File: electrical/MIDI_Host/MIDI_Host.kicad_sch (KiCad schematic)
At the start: 9 parts, among them CN1 USB-CON-AF-LCP-Offset, J1 Blackheadphonejack, J2 Blackheadphonejack, J3 USB_C_TYPE-C-32-M-12, SW1 ST-0-102-C03-N003-RS, SW2 TC-1109DE-C-G

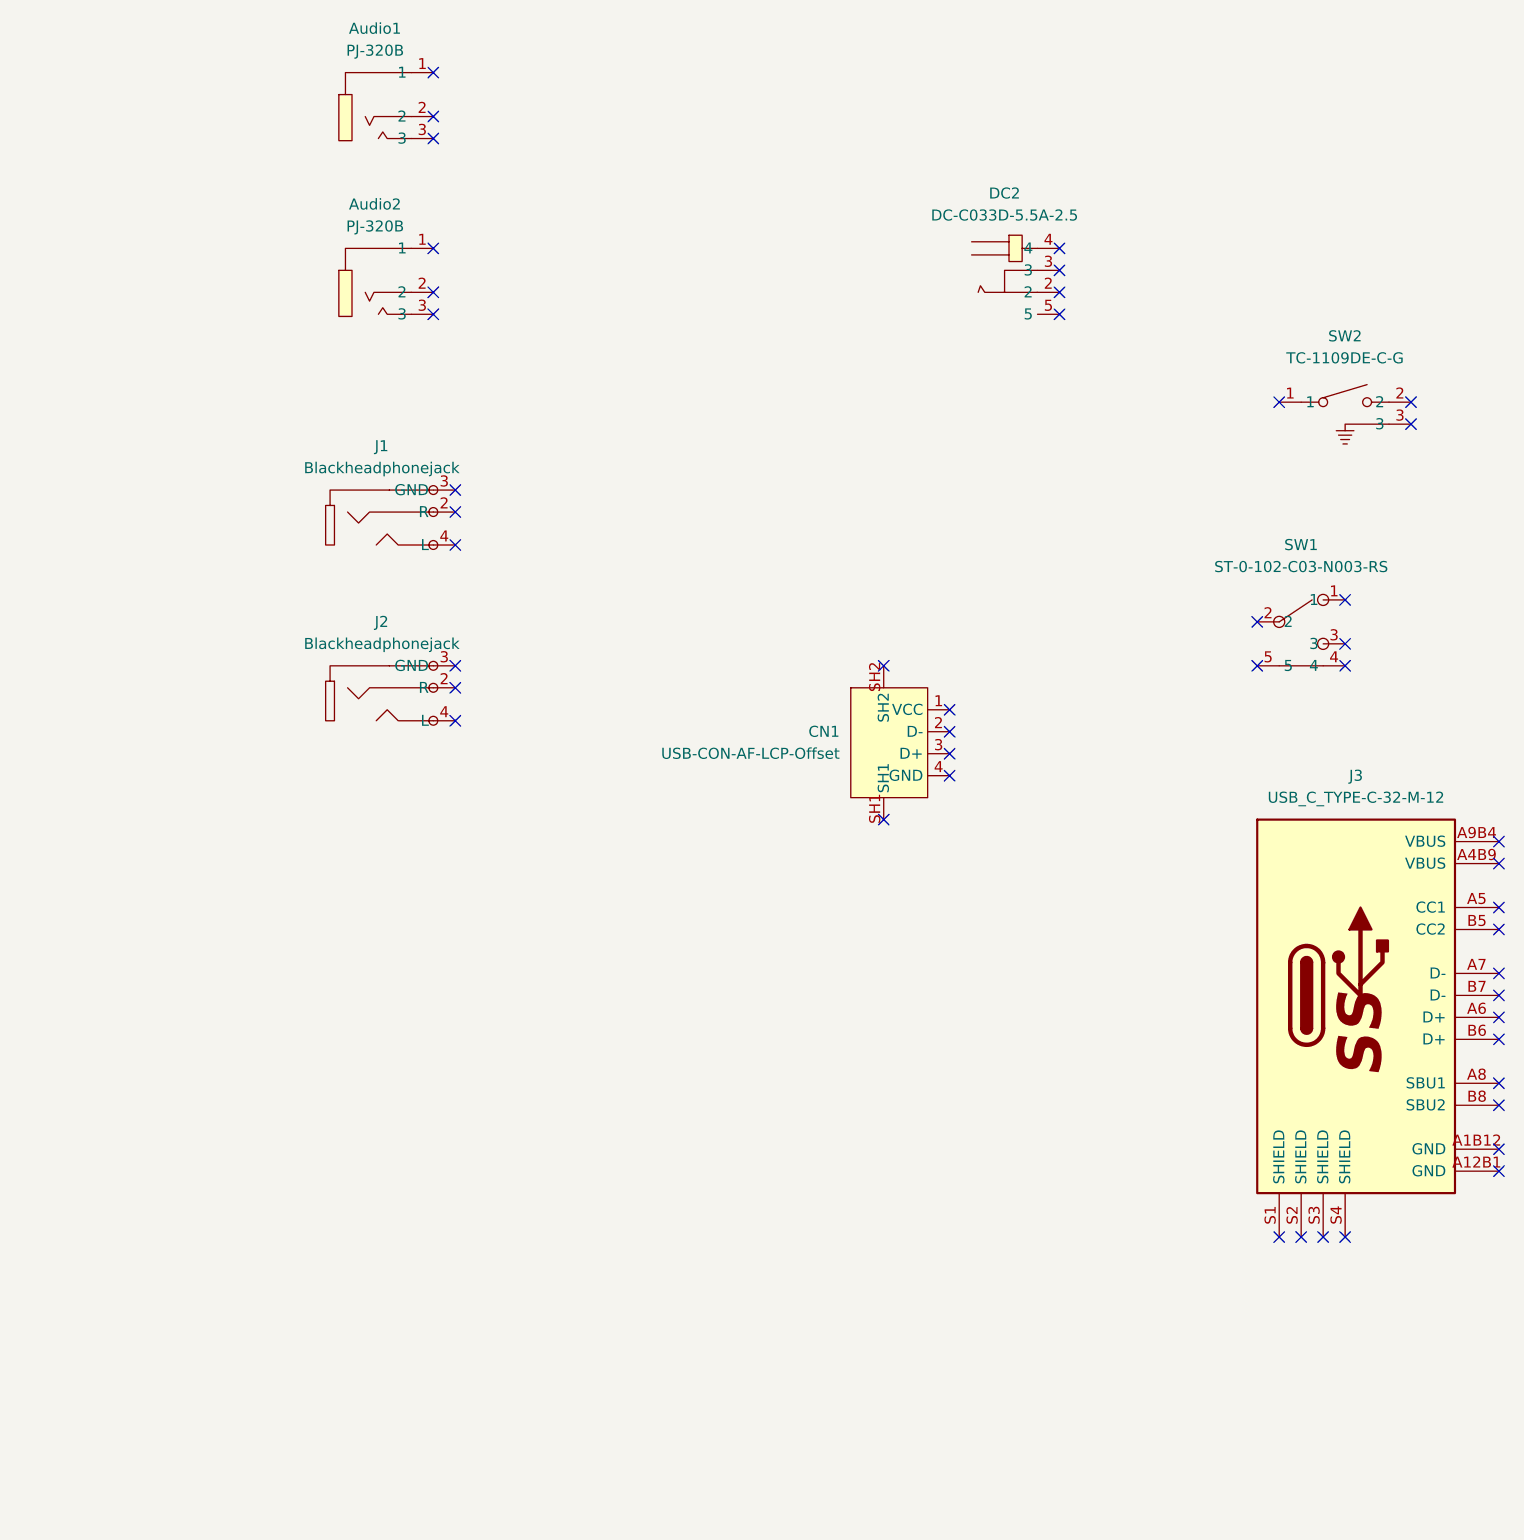
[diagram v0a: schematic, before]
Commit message: SUKU schematic progress
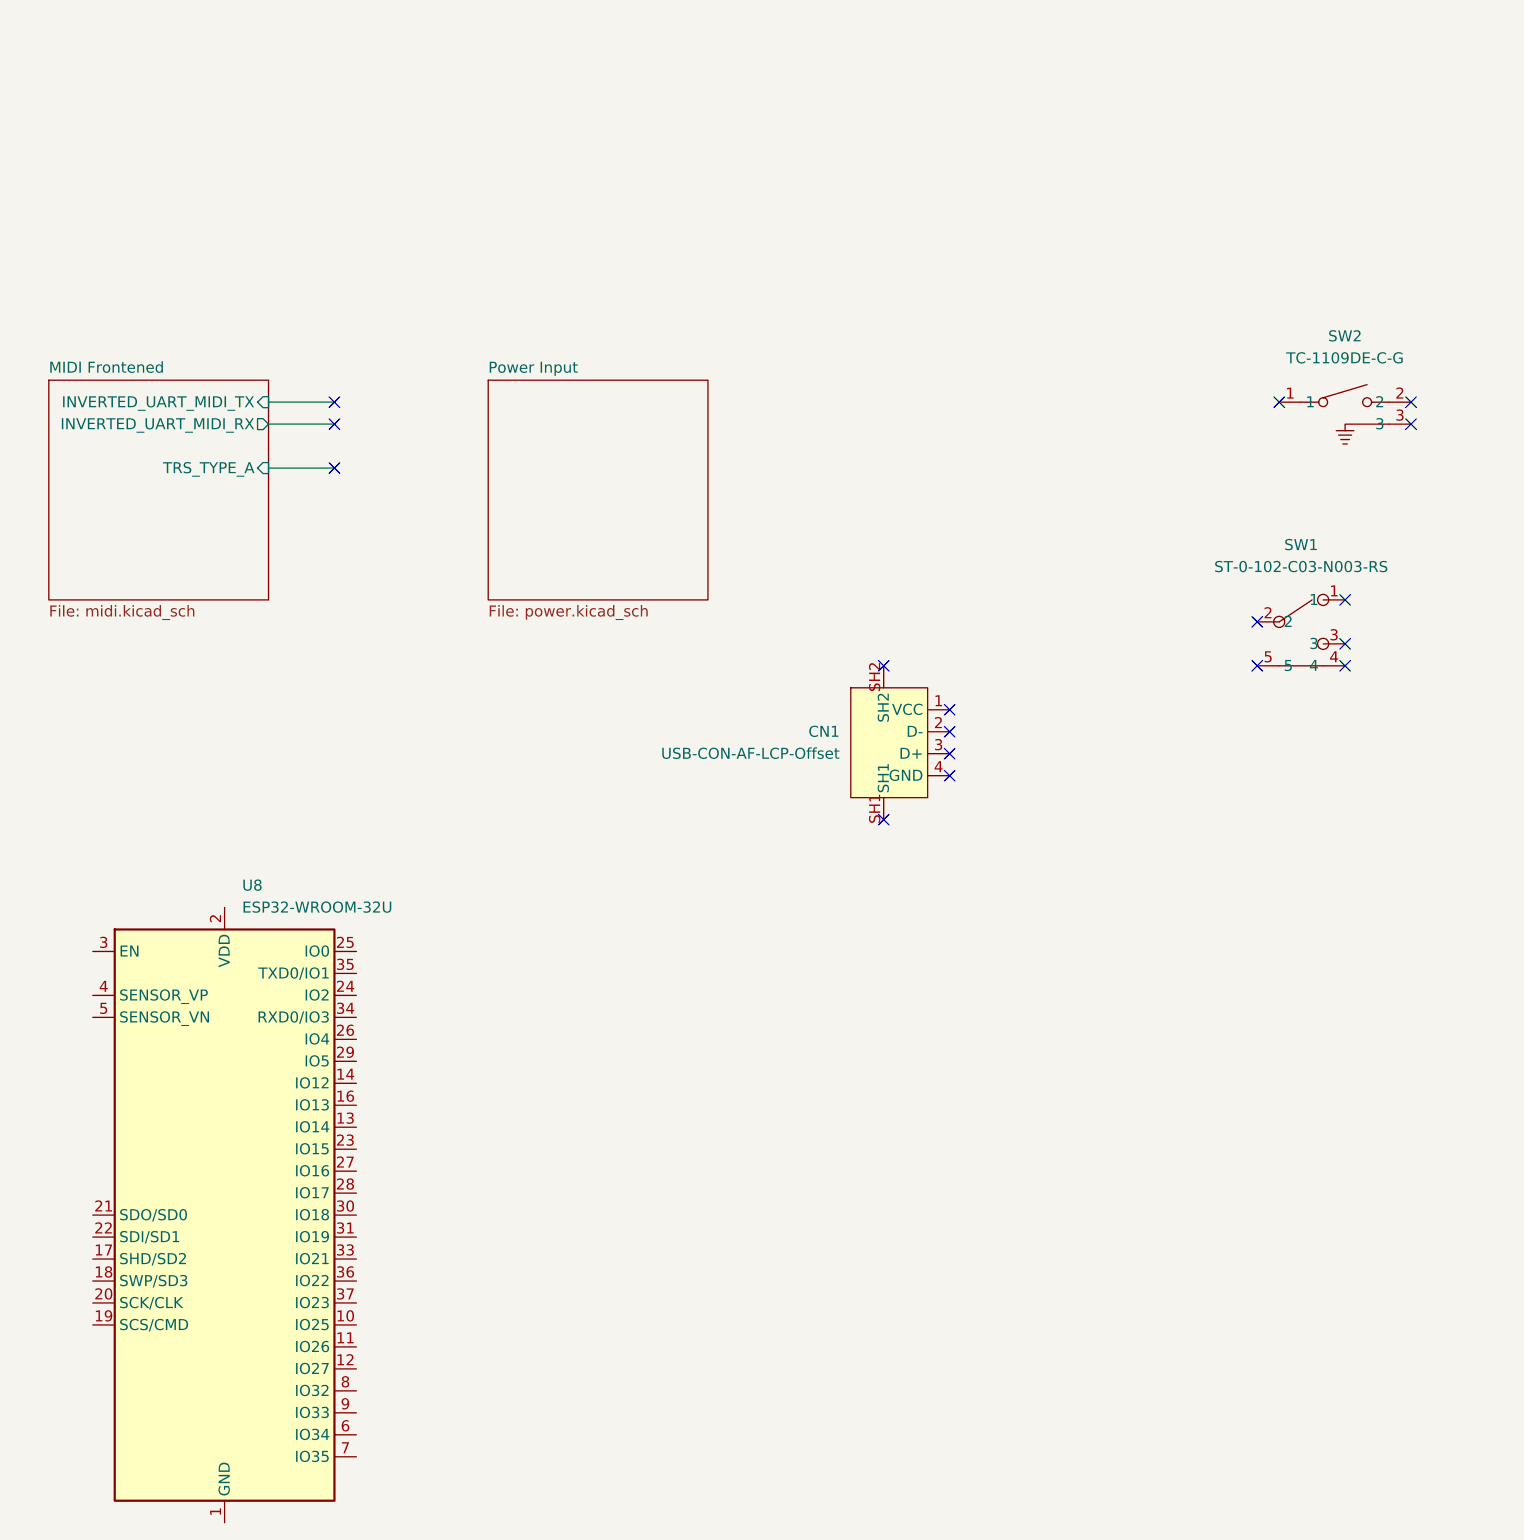
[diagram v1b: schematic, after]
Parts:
- removed Audio1, Audio2: PJ-320B, suku_basics:AUDIO-SMD_PJ-320B, symbol suku_basics:PJ-320B
- removed DC2: DC-C033D-5.5A-2.5, suku_basics:DC-IN-TH_DC-C033D-5.5A-2.5, symbol suku_basics:DC-C033D-5.5A-2.5
- removed J1, J2: Blackheadphonejack, suku_basics:AUDIO-TH_PJ-3200, symbol suku_basics:Blackheadphonejack
- removed J3: USB_C_TYPE-C-32-M-12, suku_basics:USB_C_Korean_Hroparts_TYPE-C-31-M-12, symbol suku_basics:USB_C_TYPE-C-32-M-12
- added U8: ESP32-WROOM-32U, RF_Module:ESP32-WROOM-32U, symbol RF_Module:ESP32-WROOM-32U
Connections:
- new net: U8.1 (GND), U8.15 (GND), U8.38 (GND), U8.39 (GND)
- no-connect marks 46 -> 17
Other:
- added sheet MIDI Frontened (midi.kicad_sch)
- added sheet Power Input (power.kicad_sch)

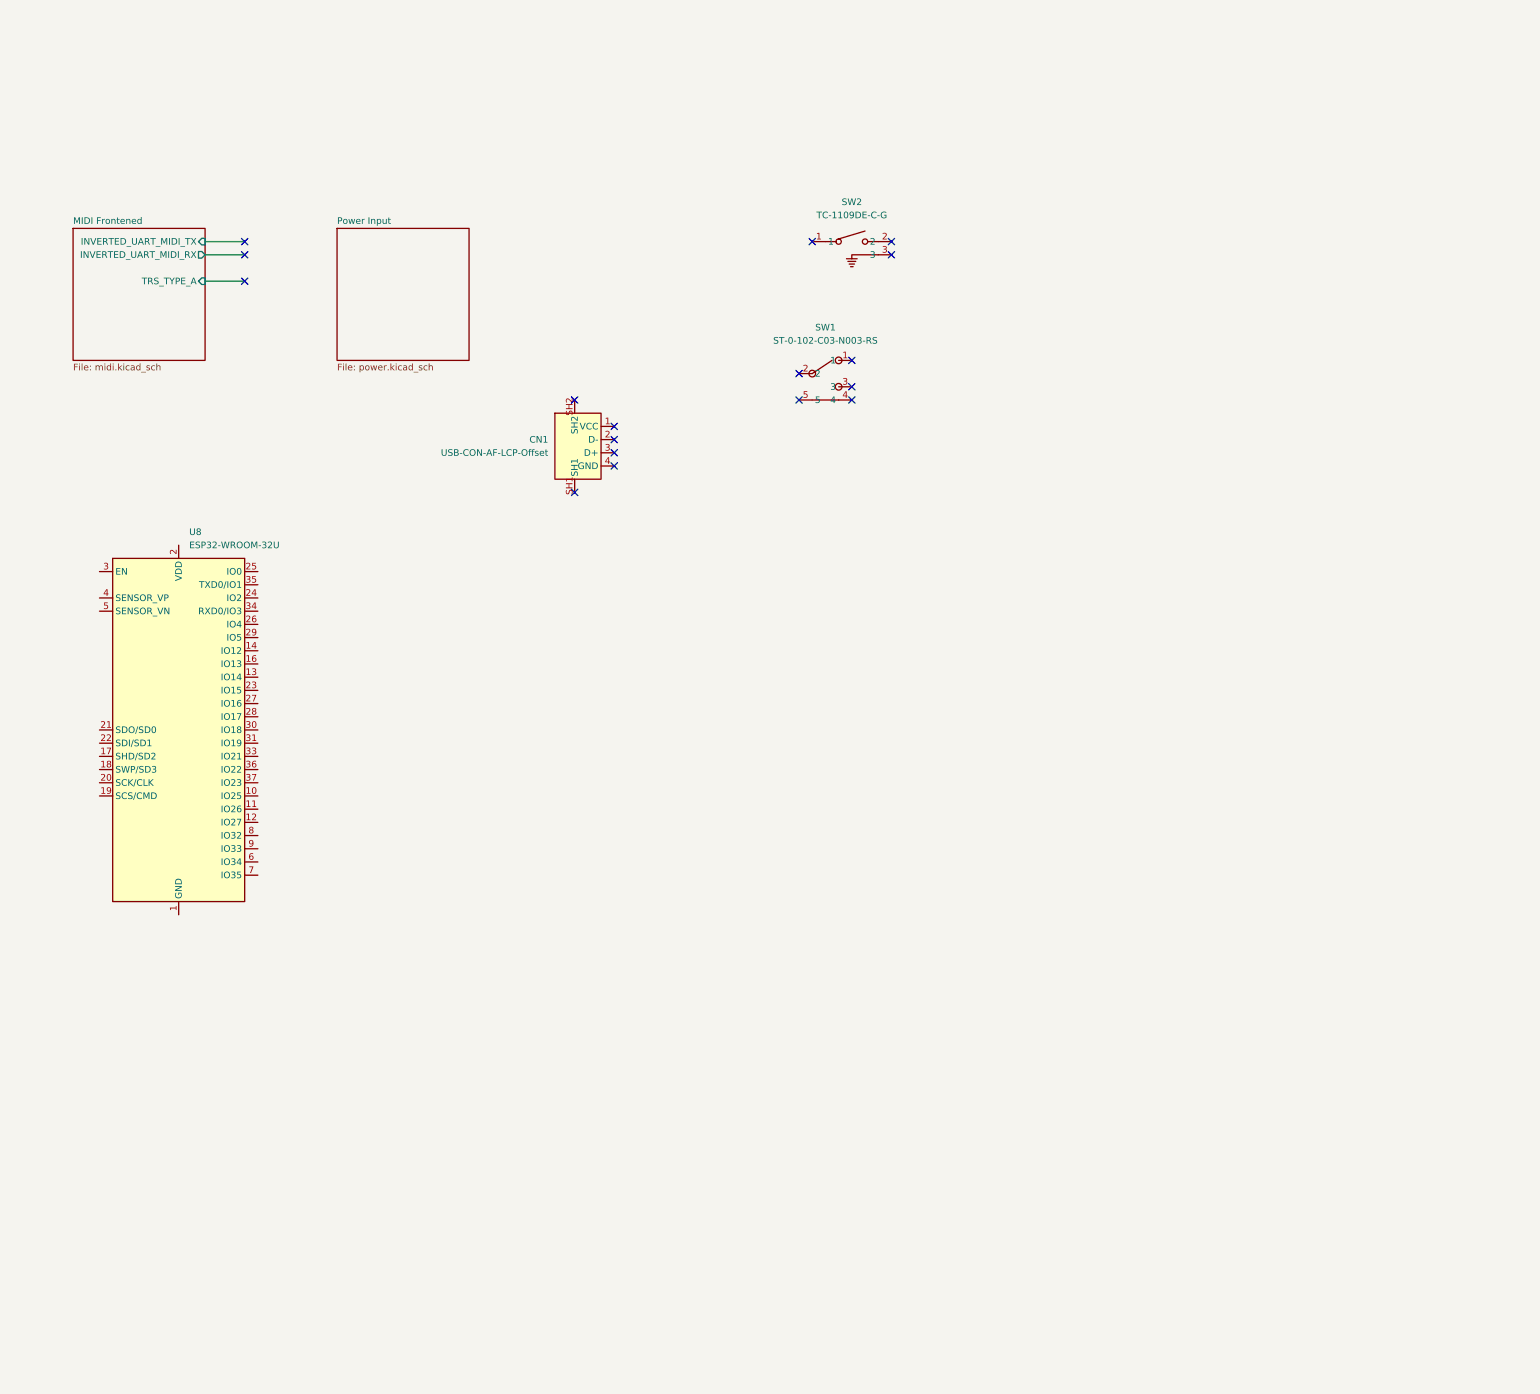
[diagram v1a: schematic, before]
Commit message: SUKU sch done
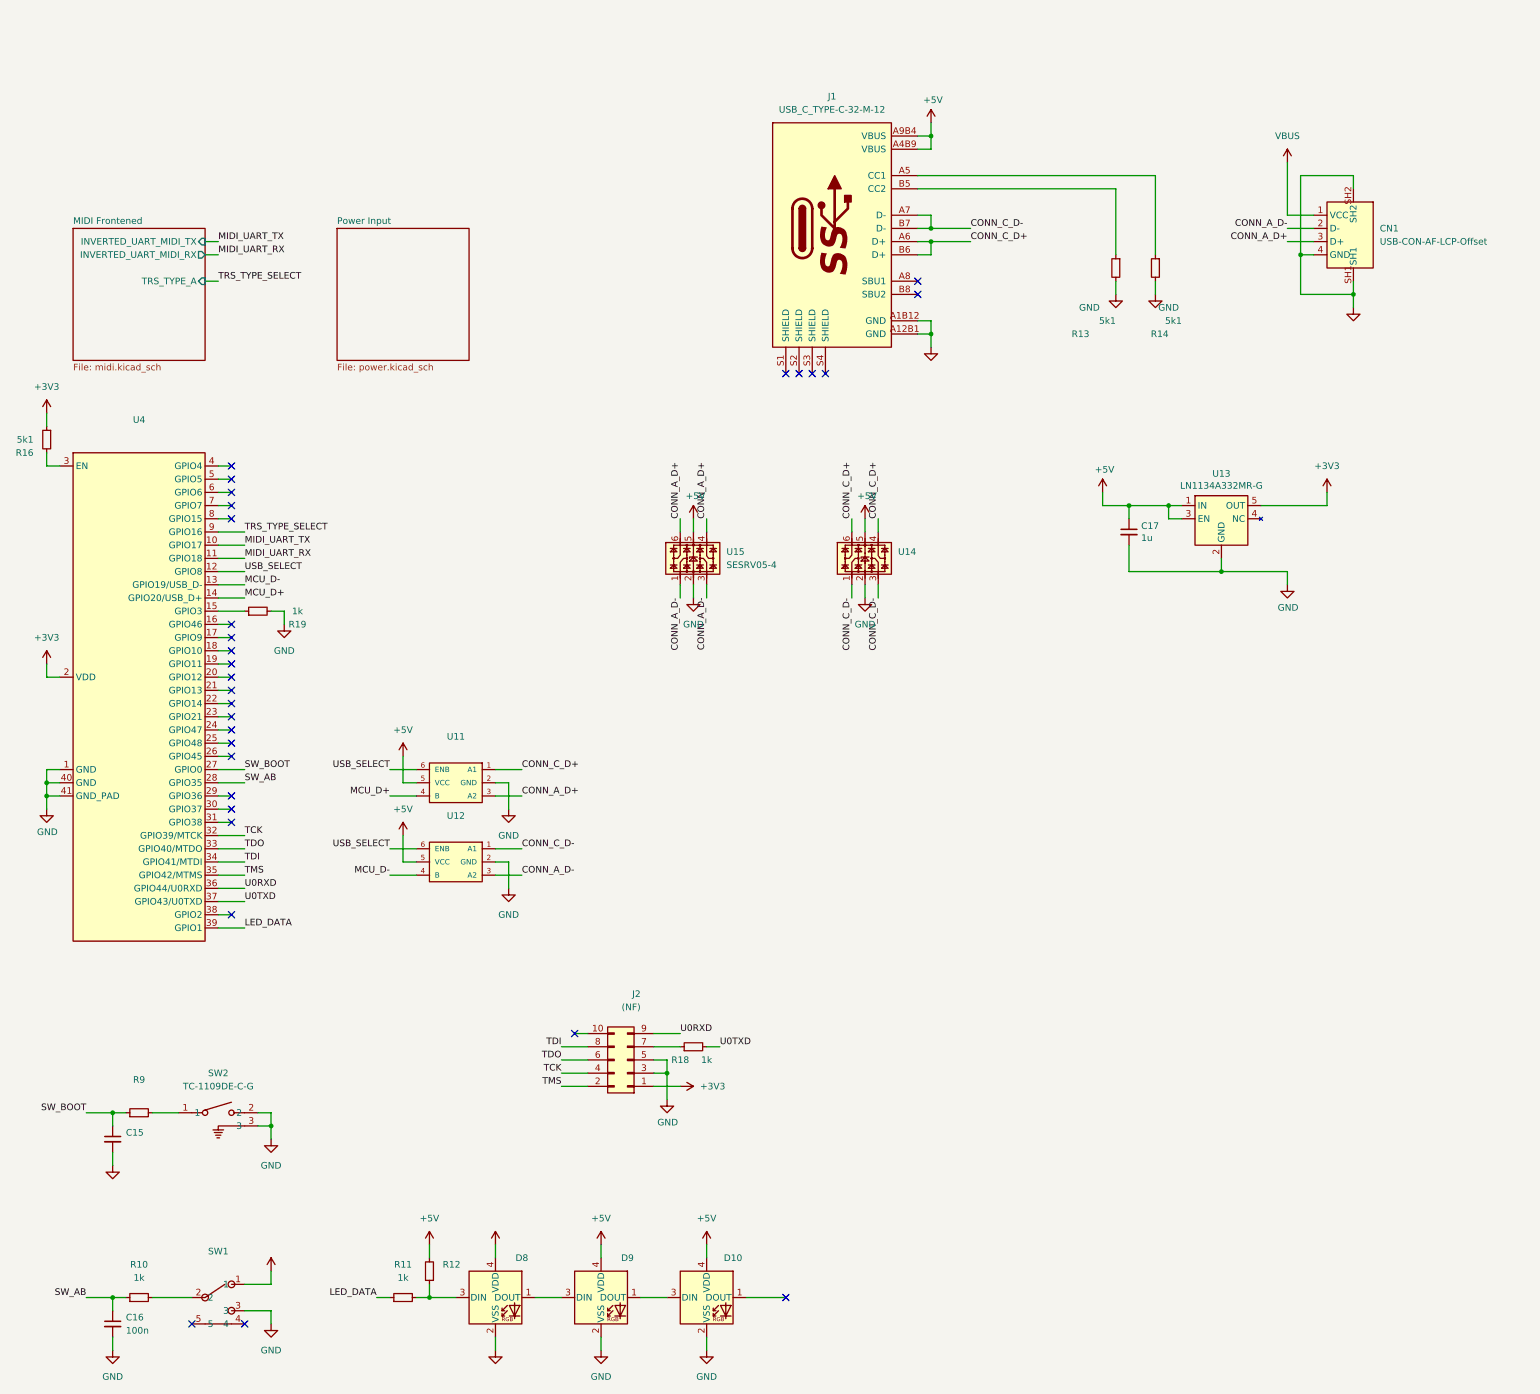
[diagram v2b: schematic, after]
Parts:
- removed U8: ESP32-WROOM-32U, RF_Module:ESP32-WROOM-32U, symbol RF_Module:ESP32-WROOM-32U
- added C15: (no value), suku_basics:CAP_0805, symbol suku_basics:CAP
- added C16: 100n, suku_basics:CAP_0805, symbol suku_basics:CAP
- added C17: 1u, suku_basics:CAP_0805, symbol suku_basics:CAP
- added D10, D8, D9: (no value), symbol suku_basics:UI_WS2812C-2020
- added J1: USB_C_TYPE-C-32-M-12, suku_basics:USB_C_Korean_Hroparts_TYPE-C-31-M-12, symbol suku_basics:USB_C_TYPE-C-32-M-12
- added J2: (NF), Connector_PinHeader_1.27mm:PinHeader_2x05_P1.27mm_Vertical, symbol Connector_Generic:Conn_02x05_Odd_Even
- added R10, R11, R18, R19: 1k, suku_basics:RES_0805, symbol suku_basics:RES
- added R12, R9: (no value), suku_basics:RES_0805, symbol suku_basics:RES
- added R13, R14, R16: 5k1, suku_basics:RES_0805, symbol suku_basics:RES
- added U11, U12: (no value), suku_basics:SOT-363_SC-70-6, symbol suku_basics:BL1551B
- added U13: LN1134A332MR-G, suku_basics:SOT-23-5, symbol suku_basics:U_REGULATOR_SOT23-5
- added U14: (no value), suku_basics:SOT-23-6, symbol suku_basics:U_ESD_4ch
- added U15: SESRV05-4, suku_basics:SOT-23-6, symbol suku_basics:U_ESD_4ch
- added U4: (no value), suku_basics:ESP32-S3-WROOM-1U, symbol suku_basics:ESP32-S3-WROOM-1U
- SW1: value ST-0-102-C03-N003-RS -> (none)
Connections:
- net +3V3: now reaches SW1.1
- net +3V3: now also J2.1 (Pin_1), R16.1, U13.5 (OUT), U4.2 (VDD)
- net at SW1.2: now also R10.2
- net GND: now reaches SW1.3
- net GND: now also CN1.4 (GND), CN1.SH1, CN1.SH2, SW2.2, SW2.3, C15.2, C16.2, C17.2, D10.2 (VSS), D8.2 (VSS), D9.2 (VSS), J1.A12B1 (GND), J1.A1B12 (GND), J2.3 (Pin_3), J2.5 (Pin_5), R13.2, R14.2, R19.2, U11.2 (GND), U12.2 (GND), U13.2 (GND), U14.2, U15.2, U4.1 (GND), U4.40 (GND), U4.41 (GND_PAD)
- net at SW2.1: now also R9.2
- net VBUS: now reaches CN1.1 (VCC)
- net CONN_A_D-: now reaches CN1.2 (D-)
- net CONN_A_D-: now also U12.3 (A2), U15.1, U15.3
- net CONN_A_D+: now reaches CN1.3 (D+)
- net CONN_A_D+: now also U11.3 (A2), U15.4, U15.6
- new net: J2.7 (Pin_7), R18.1
- new net: D8.3 (DIN), R11.2, R12.1
- new net: R19.1, U4.15 (GPIO3)
- new net: R16.2, U4.3 (EN)
- new net: D10.3 (DIN), D9.1 (DOUT)
- new net: D8.1 (DOUT), D9.3 (DIN)
- new net: J1.A5 (CC1), R14.1
- new net: J1.B5 (CC2), R13.1
- new net +5V: C17.1, D10.4 (VDD), D8.4 (VDD), D9.4 (VDD), J1.A4B9 (VBUS), J1.A9B4 (VBUS), R12.2, U11.5 (VCC), U12.5 (VCC), U13.1 (IN), U13.3 (EN), U14.5, U15.5
- new net CONN_C_D+: J1.A6 (D+), J1.B6 (D+), U11.1 (A1), U14.4, U14.6
- new net CONN_C_D-: J1.A7 (D-), J1.B7 (D-), U12.1 (A1), U14.1, U14.3
- new net LED_DATA: R11.1, U4.39 (GPIO1)
- new net MCU_D+: U11.4 (B), U4.14 (GPIO20/USB_D+)
- new net MCU_D-: U12.4 (B), U4.13 (GPIO19/USB_D-)
- new net MIDI_UART_RX: U4.11 (GPIO18)
- new net MIDI_UART_TX: U4.10 (GPIO17)
- new net SW_AB: C16.1, R10.1, U4.28 (GPIO35)
- new net SW_BOOT: C15.1, R9.1, U4.27 (GPIO0)
- new net TCK: J2.4 (Pin_4), U4.32 (GPIO39/MTCK)
- new net TDI: J2.8 (Pin_8), U4.34 (GPIO41/MTDI)
- new net TDO: J2.6 (Pin_6), U4.33 (GPIO40/MTDO)
- new net TMS: J2.2 (Pin_2), U4.35 (GPIO42/MTMS)
- new net TRS_TYPE_SELECT: U4.9 (GPIO16)
- new net U0RXD: J2.9 (Pin_9), U4.36 (GPIO44/U0RXD)
- new net U0TXD: R18.2, U4.37 (GPIO43/U0TXD)
- new net USB_SELECT: U11.6 (ENB), U12.6 (ENB), U4.12 (GPIO8)
- no-connect marks 17 -> 30
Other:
- moved on the sheet: CN1, SW1, SW2
